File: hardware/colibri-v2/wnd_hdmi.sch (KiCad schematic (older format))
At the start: 13 parts

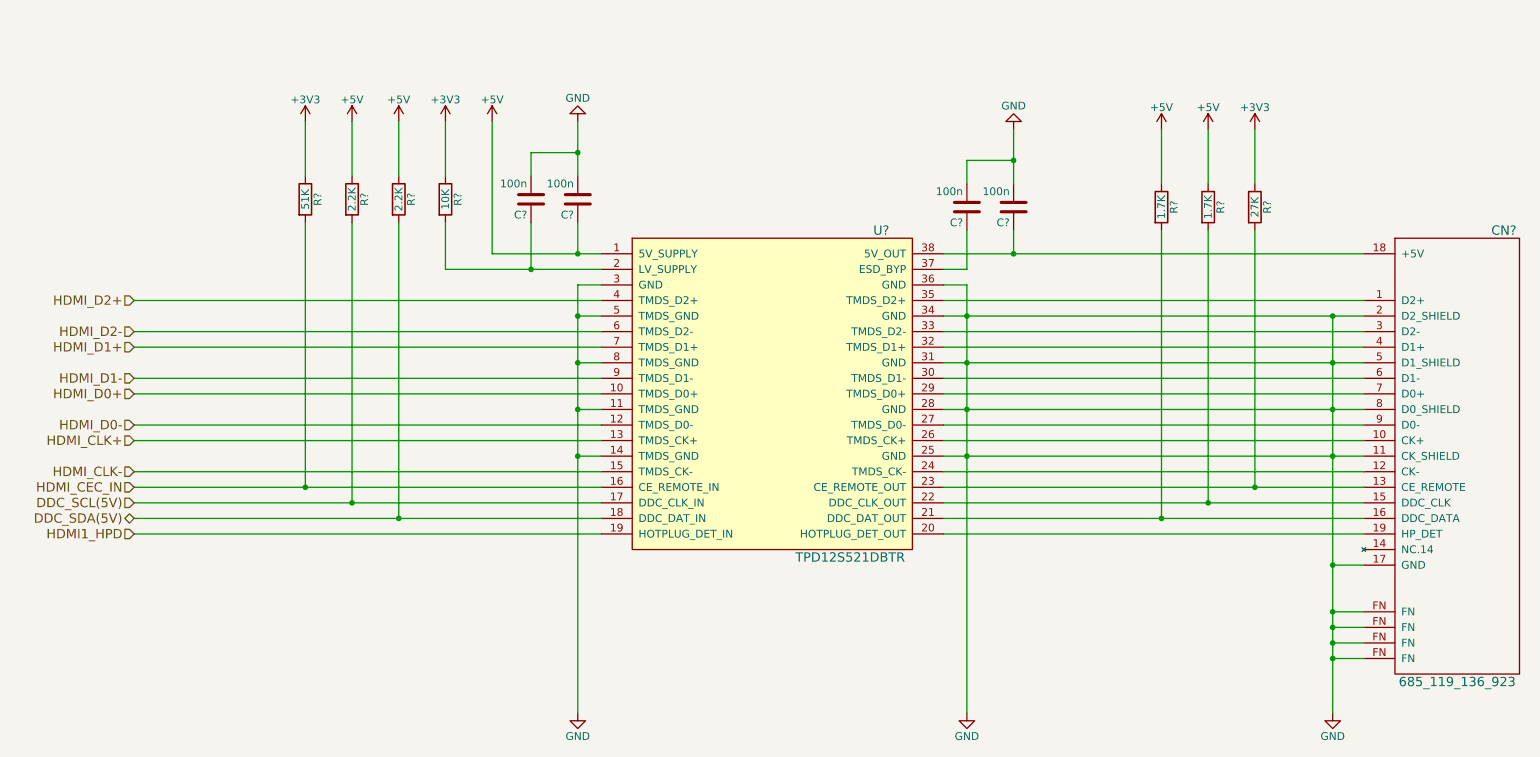
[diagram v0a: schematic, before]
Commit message: Work on the Cortex sheet
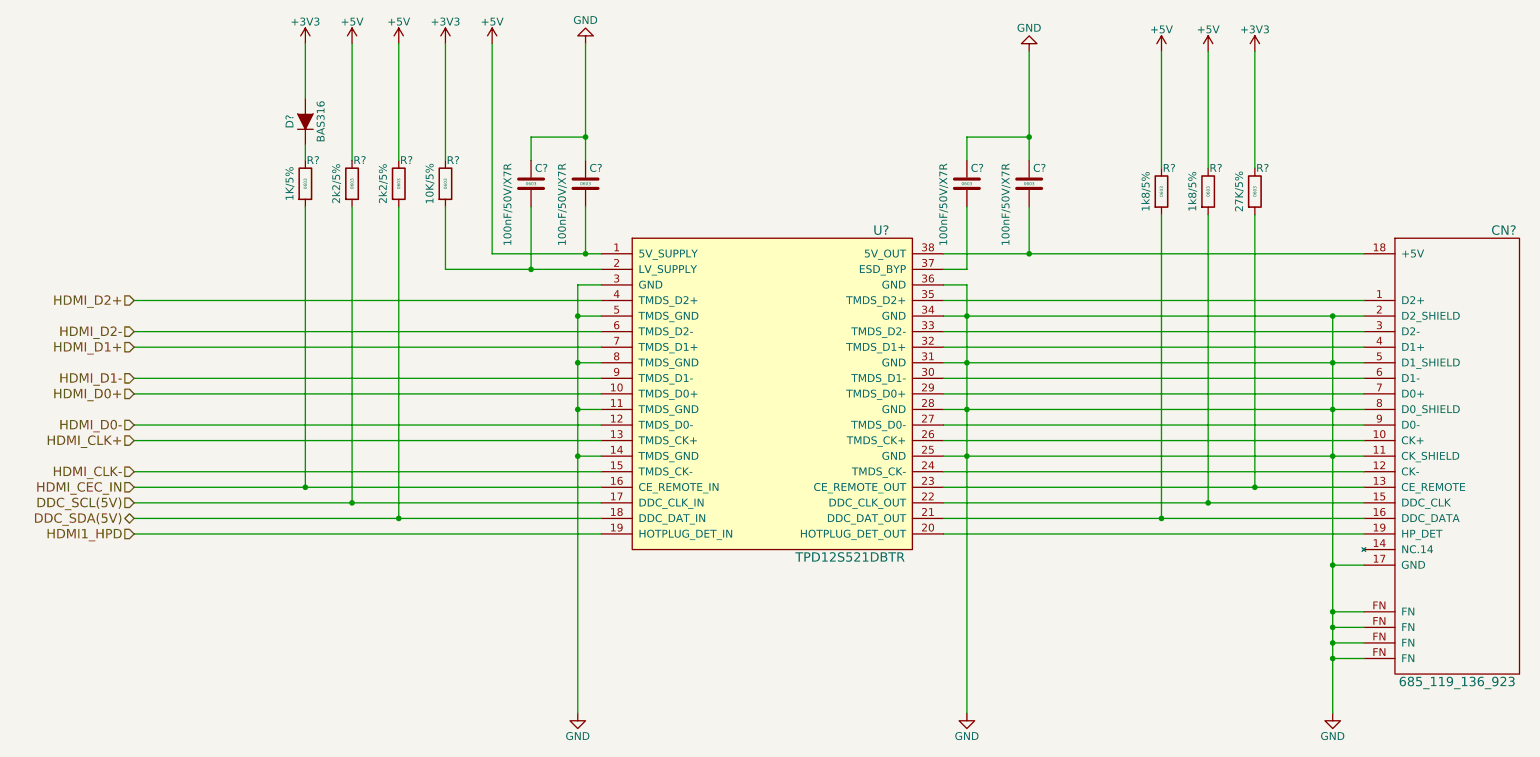
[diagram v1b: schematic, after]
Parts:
- removed C? (x4): 100n, symbol C
- removed R? (x2): 1.7K, Resistors_SMD:R_0603, symbol R
- removed R?: 27K, Resistors_SMD:R_0603, symbol R
- removed R?: 10K, Resistors_SMD:R_0603, symbol R
- removed R? (x2): 2.2K, Resistors_SMD:R_0603, symbol R
- removed R?: 51K, Resistors_SMD:R_0603, symbol R
- added C? (x4): 100nF/50V/X7R, Capacitors_SMD:C_0603, symbol C_SMT
- added D?: BAS316, Diodes_SMD:SOD-323, symbol D_SMT
- added R?: 10K/5%, Resistors_SMD:R_0603, symbol R_SMT
- added R? (x2): 2k2/5%, Resistors_SMD:R_0603, symbol R_SMT
- added R?: 1K/5%, Resistors_SMD:R_0603, symbol R_SMT
- added R? (x2): 1k8/5%, Resistors_SMD:R_0603, symbol R_SMT
- added R?: 27K/5%, Resistors_SMD:R_0603, symbol R_SMT
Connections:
- net +3V3: now also D?.2 (A), R?.1, R?.1
- net +5V: now also C?.2, R?.1, R?.1, R?.1, R?.1
- net DDC_SCL(5V): now also R?.2
- net DDC_SDA(5V): now also R?.2
- net GND: now also C?.1, C?.1, C?.1, C?.1
- net HDMI_CEC_IN: now also R?.2
- net at U?.2 (LV_SUPPLY): now also C?.2, R?.2
- net at CN?.16 (DDC_DATA), U?.21 (DDC_DAT_OUT): now also R?.2
- net at CN?.15 (DDC_CLK), U?.22 (DDC_CLK_OUT): now also R?.2
- net at CN?.13 (CE_REMOTE), U?.23 (CE_REMOTE_OUT): now also R?.2
- net at U?.37 (ESD_BYP): now also C?.2
- net at CN?.18 (+5V), U?.38 (5V_OUT): now also C?.2
- new net: D?.1 (K), R?.1
